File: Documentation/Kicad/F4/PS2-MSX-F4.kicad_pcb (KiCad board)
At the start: 2 copper layers, 55 x 65 mm, 34 parts, among them J1 Conn_02x17_Odd_Even, J2 Conn_01x04, J3 Conn_01x04, Q1 2SC1815, Q2 2N2907, U1 WeAct Studio STM32F401CEU6 V3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

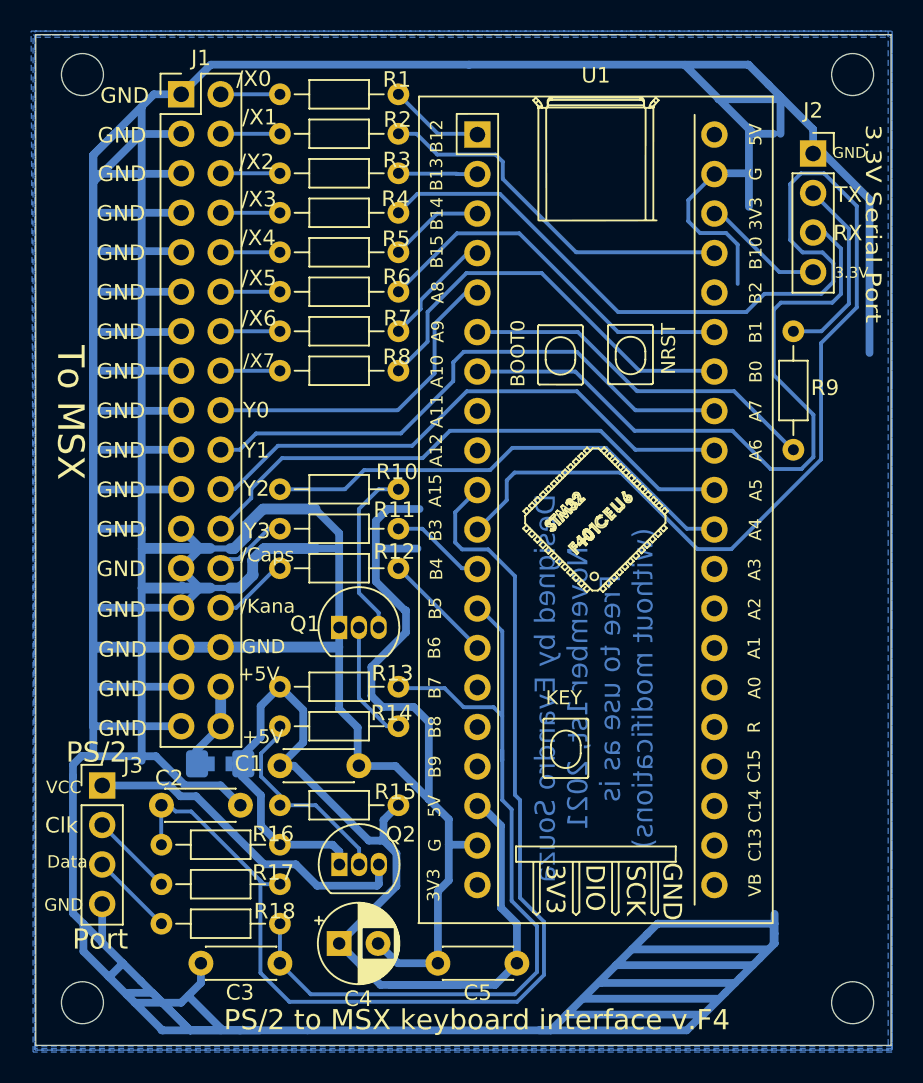
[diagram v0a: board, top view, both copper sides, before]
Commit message: Kicad schematic and PCB files
Kicad schematic and PCB files upload
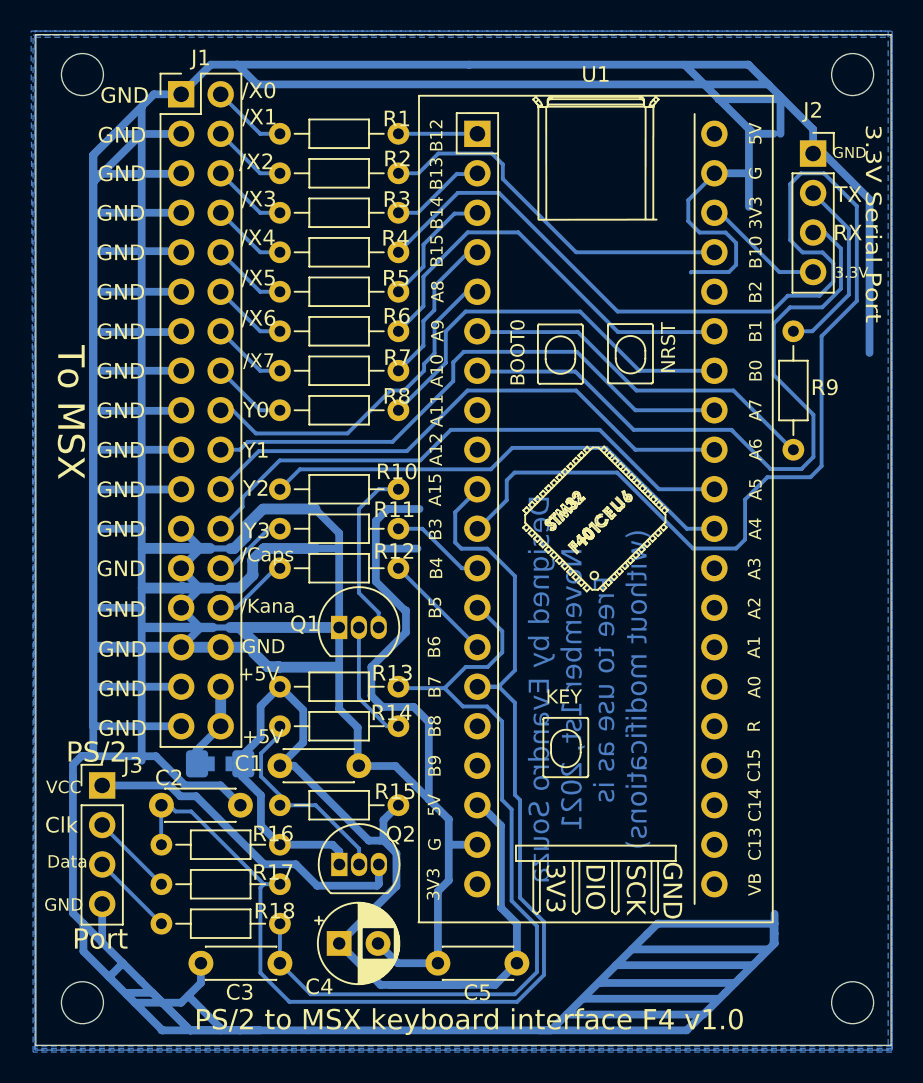
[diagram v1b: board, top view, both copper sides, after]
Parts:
- moved R2 2.54 mm to (139.7, 81.3)
- moved R4 2.54 mm to (139.7, 86.4)
- moved R5 2.54 mm to (139.7, 88.9)
- moved R7 2.54 mm to (139.7, 94.0)
- moved R1 2.54 mm to (139.7, 78.7)
- moved R3 2.54 mm to (139.7, 83.8)
- moved R6 2.54 mm to (139.7, 91.4)
- moved R8 2.54 mm to (139.7, 96.5)
- moved U1 0.05 mm to (152.4, 78.7)
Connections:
- net Net-(R1-Pad2) renamed /X0'
- U1 pad 15: Net-(U1-Pad15) -> /PS2Clk
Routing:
- net GNDD: track 586.7 -> 638.9 mm
- net /X3': track 92.1 -> 94.9 mm
- net /PS2Clk: track 73.7 -> 76.2 mm
- net /X6': track 7.70 -> 10.2 mm
- net /X4': track 6.06 -> 8.33 mm
- net /X5': track 24.6 -> 26.9 mm
- net /X6: track 3.81 -> 4.86 mm
- net /X4: track 3.81 -> 4.86 mm
- net /X3: track 3.81 -> 4.86 mm
- net /X1: track 3.81 -> 4.86 mm
- net /X7: track 3.81 -> 4.86 mm
- net /X5: track 3.81 -> 4.86 mm
- net /X2: track 3.81 -> 4.86 mm
- net /X0': track 6.20 -> 5.14 mm
- net /X0: track 3.81 -> 4.86 mm
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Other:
- net class Default added: clearance 0.2, trace_width 0.25, via_dia 0.8, via_drill 0.4
- board text added: "PS/2 to MSX keyboard interface F4 v1.0"
- board text removed: "PS/2 to MSX keyboard interface v.F4"
